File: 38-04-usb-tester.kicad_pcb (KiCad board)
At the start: 2 copper layers, 131.7 x 103.7 mm, 63 parts, among them J1 Conn_1x05, J2 USB_C_12401832E402A, J3 USB_C_12401832E402A, J4 USB_Micro-B_KH-MICRO5P-JN, J5 USB_Mini-B_U-M-M5DD-W-1, J6 USB3_A_HC-USB3.0-L168-WP, SW1 SW_SPDT, SW2 ZX-1.27BM-4PSMD, U1 STM32C031K6Tx

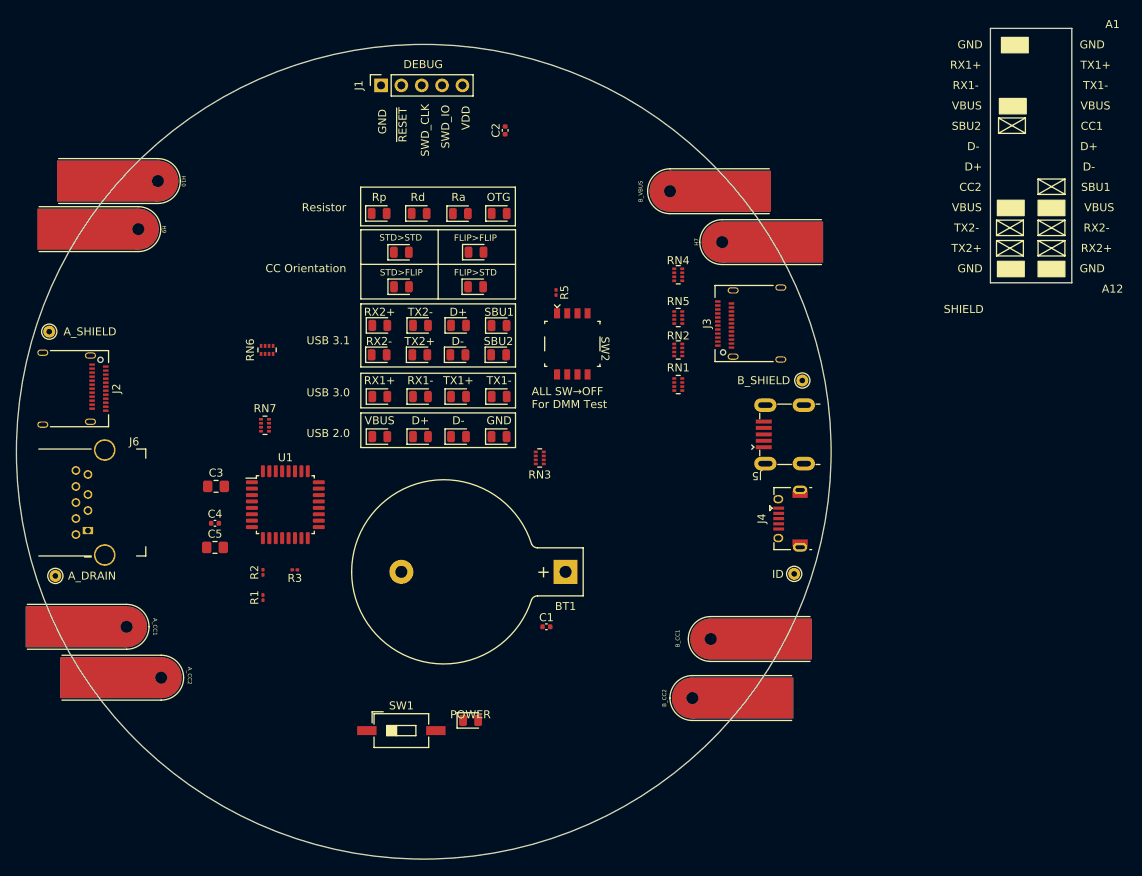
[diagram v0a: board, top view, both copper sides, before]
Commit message: pre commit to importing template
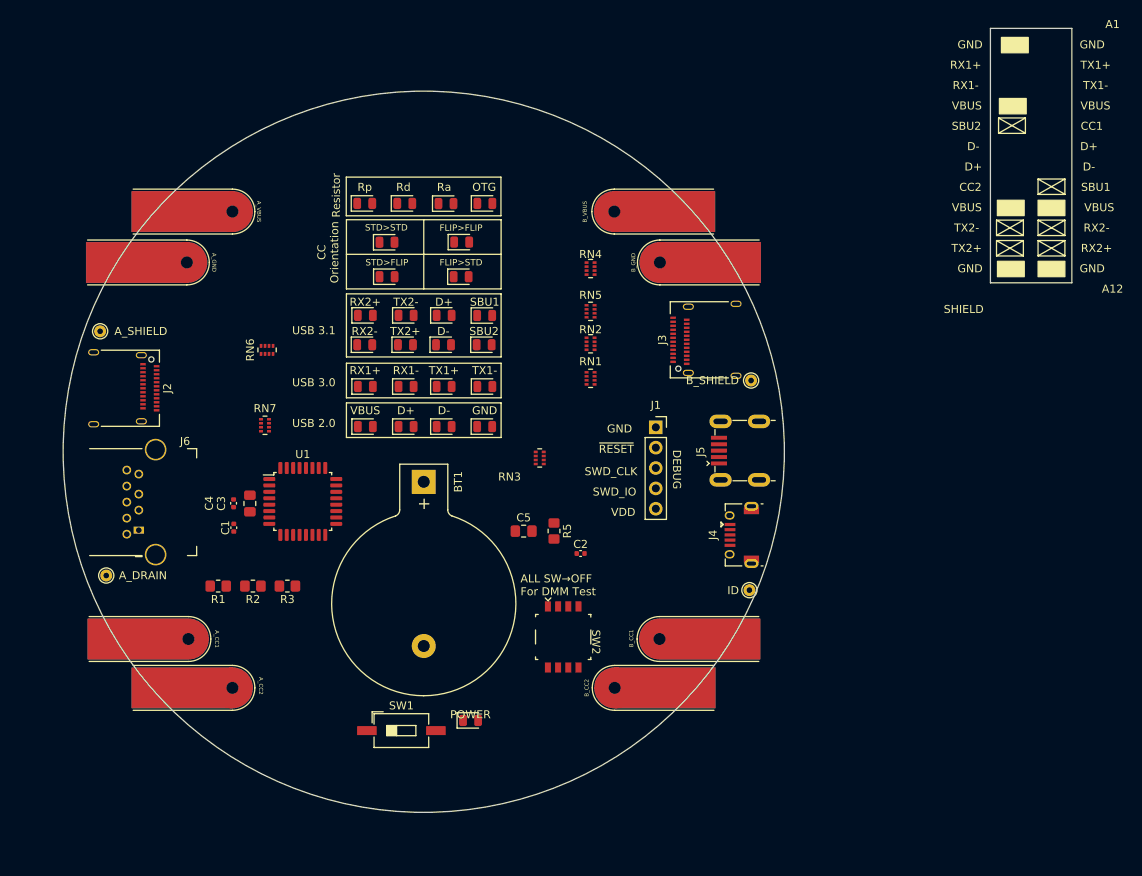
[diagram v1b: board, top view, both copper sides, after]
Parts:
- R1, R2, R3, R5: footprint Resistor_SMD:R_0201_0603Metric -> Resistor_SMD:R_0805_2012Metric_Pad1.20x1.40mm_HandSolder
- moved J1 54.7 mm to (183.9, 107.4), turned to 0 degrees
- moved C2 53.6 mm to (174.5, 123.2), turned to 0 degrees
- moved C1 40.9 mm to (131.2, 120.0), turned to -90 degrees
- moved C5 38.6 mm to (167.4, 120.4)
- moved SW2 36.6 mm to (172.3, 133.6)
- moved R5 29.8 mm to (171.2, 120.4)
- moved BT1 21.0 mm to (154.9, 114.2), turned to -90 degrees
- moved RN1 11.0 mm to (175.8, 101.3)
- moved RN2 11.0 mm to (175.8, 97.0)
- moved RN4 11.0 mm to (175.8, 87.6)
- moved RN5 11.0 mm to (175.8, 93.0)
- moved H10 10.1 mm to (118.5, 80.5)
- moved H2 9.78 mm to (191.3, 140.0)
- moved H5 8.98 mm to (118.5, 140.0)
- moved H7 8.18 mm to (196.9, 86.9)
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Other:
- board size 131.7 x 103.7 mm -> 125.9 x 97.8 mm
